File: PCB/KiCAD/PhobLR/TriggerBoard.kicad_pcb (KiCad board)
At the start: 2 copper layers, 41.7 x 9.7 mm, 5 parts, among them J1 L, J2 R, SW1 L, SW2 R

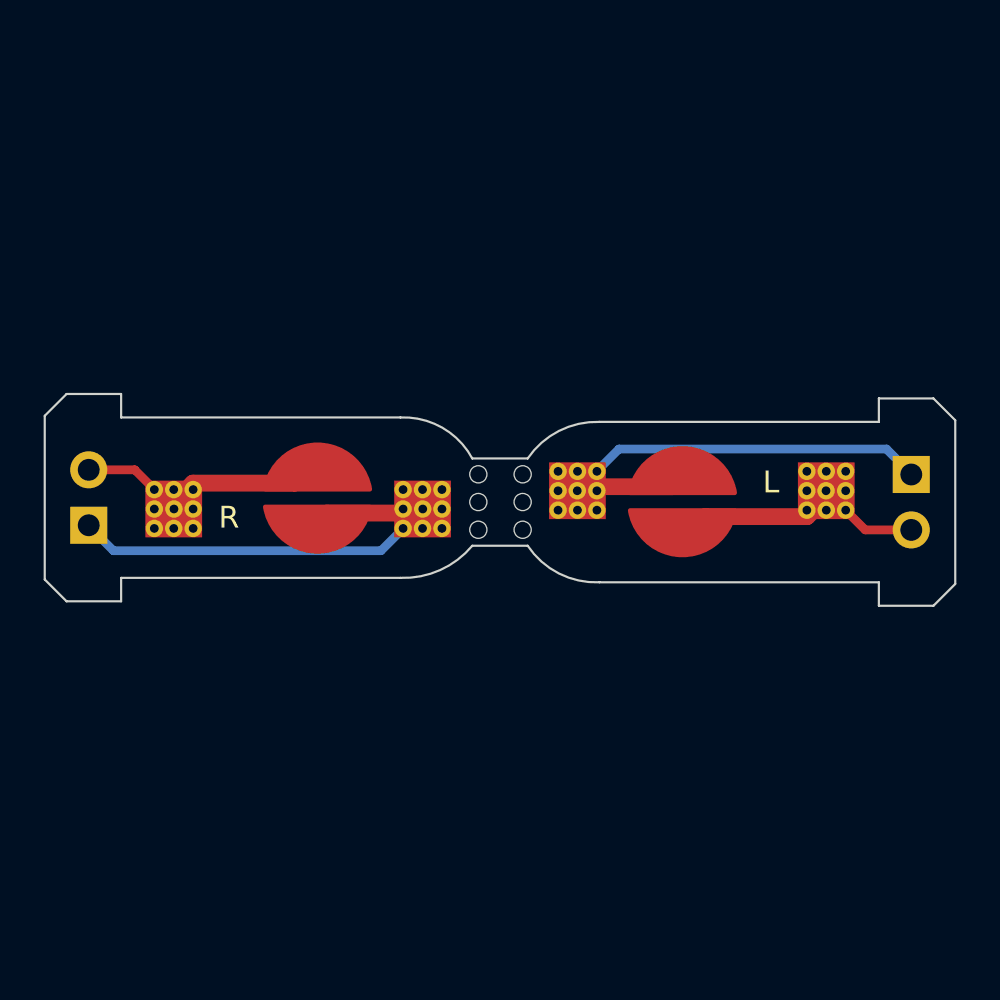
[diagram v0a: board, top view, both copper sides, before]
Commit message: push to commit
committing the push with this commit
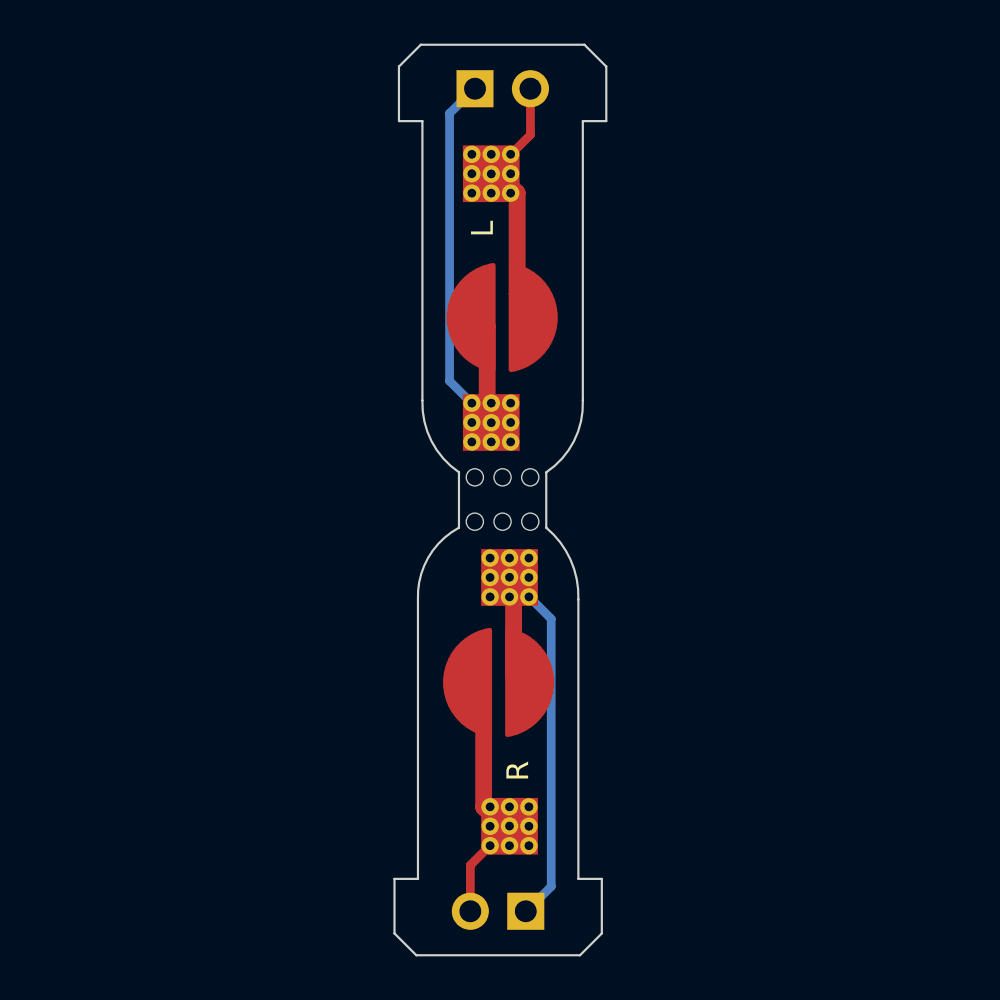
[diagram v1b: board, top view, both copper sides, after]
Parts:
- moved J2 26.7 mm to (109.6, 90.4), turned to 90 degrees
- moved J1 26.7 mm to (107.3, 52.7), turned to -90 degrees
- moved SW2 11.8 mm to (108.4, 79.9), turned to -90 degrees
- moved SW1 11.8 mm to (108.5, 63.2), turned to 90 degrees
- moved H2 1.78 mm to (108.3, 70.2), turned to 180 degrees
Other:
- board size 41.7 x 9.7 mm -> 9.7 x 41.7 mm
